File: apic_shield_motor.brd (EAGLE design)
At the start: 70.7 x 55.5 mm, 9 parts, among them U1 V_REG_7805-TO220ALT, U2 V_REG_7805-TO220ALT, U3 V_REG_7805-TO220ALT, U4 V_REG_7805-TO220ALT, U5 V_REG_7805-TO220ALT, U6 V_REG_7805-TO220ALT, U7 V_REG_7805-TO220ALT, U8 V_REG_7805-TO220ALT

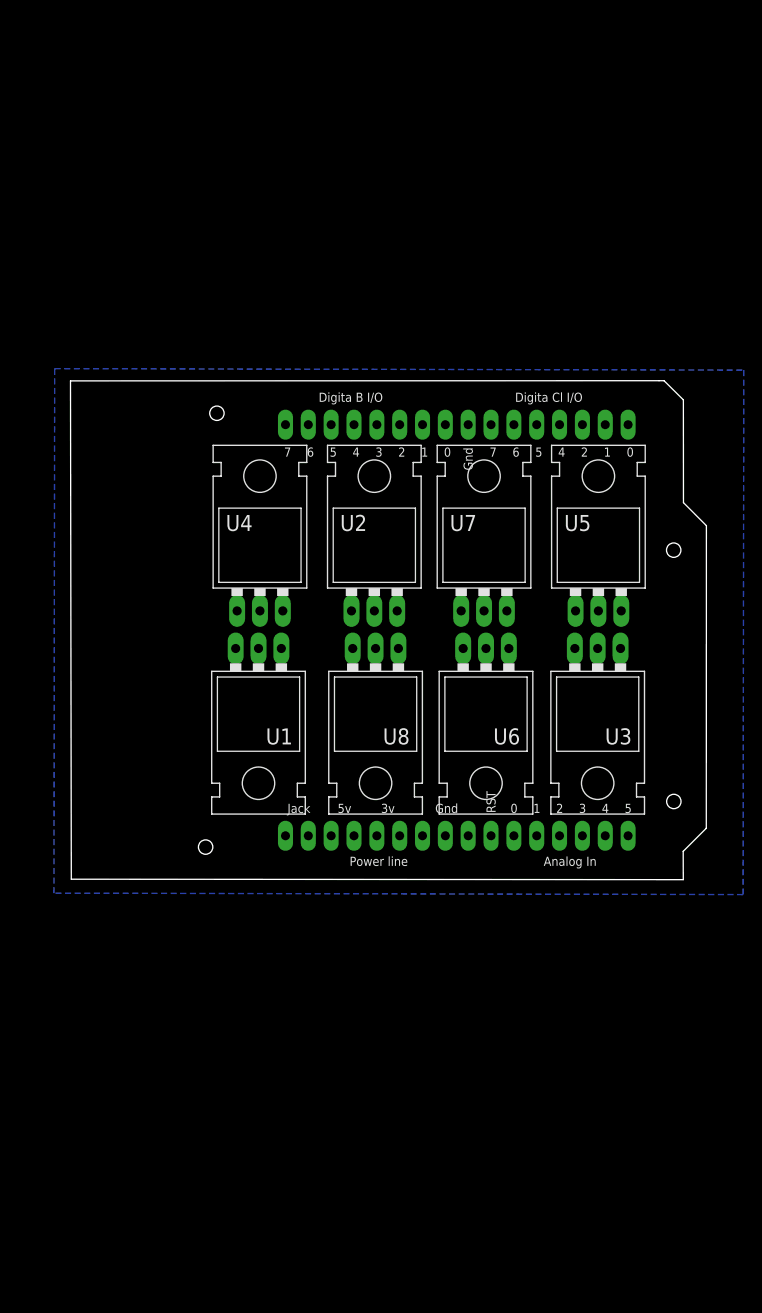
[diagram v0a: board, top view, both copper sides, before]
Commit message: update project
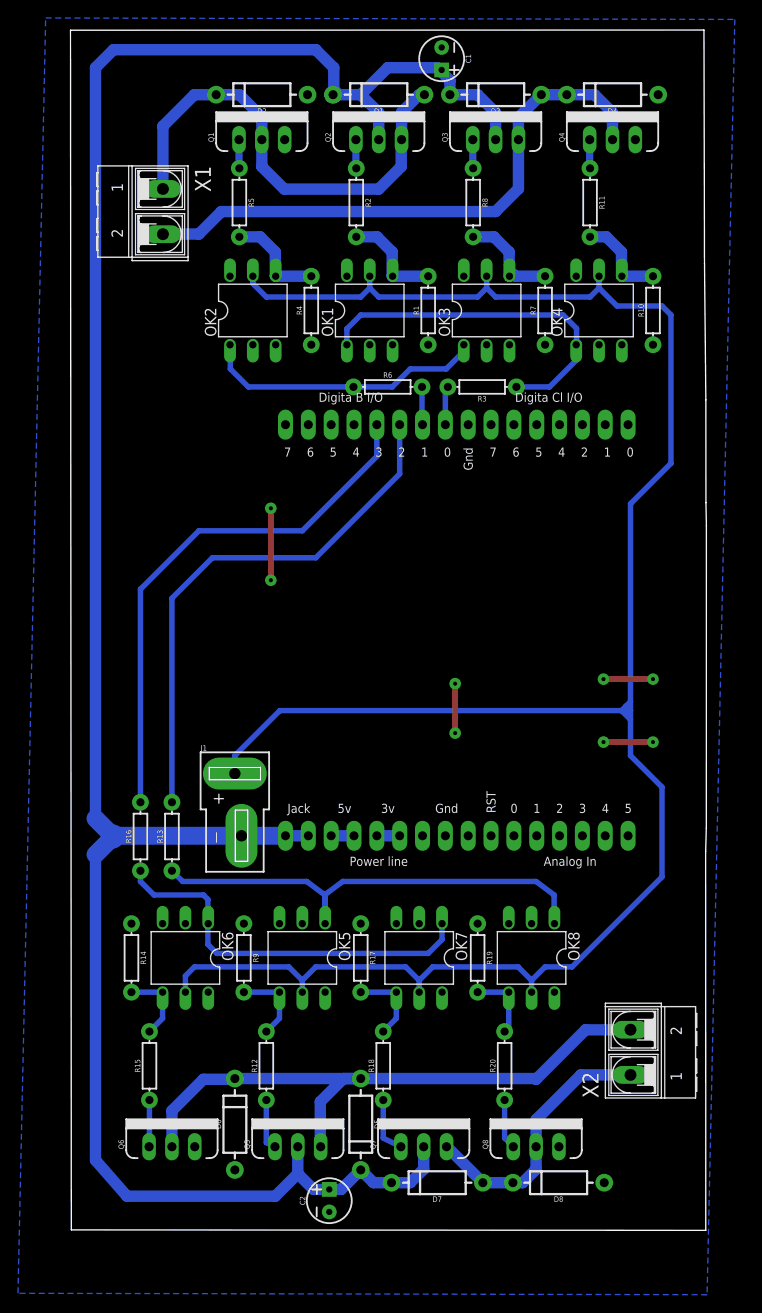
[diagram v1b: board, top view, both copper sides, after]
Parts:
- removed U1, U2, U3, U4, U5, U6, U7, U8: V_REG_7805-TO220ALT, YAEL:TO-220-ALT
- added C1, C2: 10uF, SparkFun-Capacitors:CPOL-RADIAL-2.5MM-5MM
- added D1, D2, D3, D4, D5, D6, D7, D8: 1N4004, SparkFun-DiscreteSemi:DIODE-1N4001
- added J1: (no value), SparkFun-Connectors:DEANS
- added OK1, OK2, OK3, OK4, OK5, OK6, OK7, OK8: 4N35M, optocoupler:DIL06
- added Q1, Q2, Q3, Q4, Q5, Q6, Q7, Q8: IRF540, untitled:TO220V
- added R1, R10, R14, R17, R19, R4, R7, R9: 50k, SparkFun-Resistors:AXIAL-0.3
- added R11, R12, R15, R18, R2, R20, R5, R8: 1k, SparkFun-Resistors:AXIAL-0.3
- added R13, R16, R3, R6: 330, SparkFun-Resistors:AXIAL-0.3
- added X1, X2: (no value), con-ptr500:AK500/2-H
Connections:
- new net +9V: J1.+, OK1.5, OK2.5, OK3.5, OK4.5, OK5.5, OK6.5, OK7.5, OK8.5
- new net N$1: OK1.4, R1.P$2, R2.P$2
- new net N$10: Q3.1, R8.P$1
- new net N$11: Q5.1, R12.P$1
- new net N$12: OK6.4, R14.P$2, R15.P$2
- new net N$13: OK4.4, R10.P$2, R11.P$2
- new net N$14: Q4.1, R11.P$1
- new net N$15: D3.A, D4.C, Q3.3, Q4.2, X1.2
- new net N$16: Q6.1, R15.P$1
- new net N$17: OK6.1, OK7.1, R16.P$1
- new net N$18: OK7.4, R17.P$2, R18.P$2
- new net N$19: Q7.1, R18.P$1
- new net N$2: Q2.1, R2.P$1
- new net N$20: OK8.4, R19.P$2, R20.P$2
- new net N$21: Q8.1, R20.P$1
- new net N$22: D5.A, D6.C, Q5.3, Q6.2, X2.2
- new net N$23: D7.A, D8.C, Q7.3, Q8.2, X2.1
- new net N$24: OK5.1, OK8.1, R13.P$1
- new net N$3: OK2.4, R4.P$2, R5.P$2
- new net N$4: OK1.1, OK4.1, R3.P$1
- new net N$5: Q1.1, R5.P$1
- new net N$6: OK5.4, R12.P$2, R9.P$2
- new net N$7: D1.A, D2.C, Q1.2, Q2.3, X1.1
- new net N$8: OK3.4, R7.P$2, R8.P$2
- new net N$9: OK2.1, OK3.1, R6.P$1
- net +12V: now also C1.1, C2.1, D1.C, D3.C, D5.C, D7.C, J1.-, Q2.2, Q3.2, Q5.2, Q7.2
- net GND: now also C1.2, C2.2, D2.A, D4.A, D6.A, D8.A, OK1.2, OK2.2, OK3.2, OK4.2, OK5.2, OK6.2, OK7.2, OK8.2, Q1.3, Q4.3, Q6.3, Q8.3, R1.P$1, R10.P$1, R14.P$1, R17.P$1, R19.P$1, R4.P$1, R7.P$1, R9.P$1
- net RB0: now also R3.P$2
- net RB1: now also R6.P$2
- net RB2: now also R13.P$2
- net RB3: now also R16.P$2
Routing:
- net +12V: track 0.00 -> 255.4 mm
- net +9V: track 0.00 -> 239.4 mm
- net N$22: track 0.00 -> 69.4 mm
- net N$15: track 0.00 -> 64.9 mm
- net RB3: track 0.00 -> 60.8 mm
- net RB2: track 0.00 -> 59.2 mm
- net N$24: track 0.00 -> 54.8 mm
- net N$7: track 0.00 -> 53.0 mm
- net N$17: track 0.00 -> 44.1 mm
- net N$4: track 0.00 -> 40.0 mm
- net N$9: track 0.00 -> 31.9 mm
- net N$23: track 0.00 -> 30.3 mm
- net GND: track 0.00 -> 24.5 mm, vias 0 -> 8
- net N$8: track 0.00 -> 11.5 mm
- net N$1: track 0.00 -> 11.4 mm
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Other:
- board size 70.7 x 55.5 mm -> 70.7 x 133.5 mm
